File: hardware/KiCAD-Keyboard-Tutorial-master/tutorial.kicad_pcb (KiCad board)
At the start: 2 copper layers, 185.7 x 106 mm, 51 parts, among them SW0:0 CTRL, SW0:1 SUPER, SW0:2 ALT, SW0:4 SPACE, SW1:1 SHIFT, SW1:2 Z, SW1:3 X, SW1:4 C, SW2:0 CAPS, SW2:1 A, SW2:2 S, SW2:3 D, SW2:4 F, SW3:0 TAB, SW3:1 Q, SW3:2 W, SW3:3 E, SW3:4 R, SW4:0 TILDE, SW4:1 1, SW4:2 2, SW4:3 3, SW4:4 4

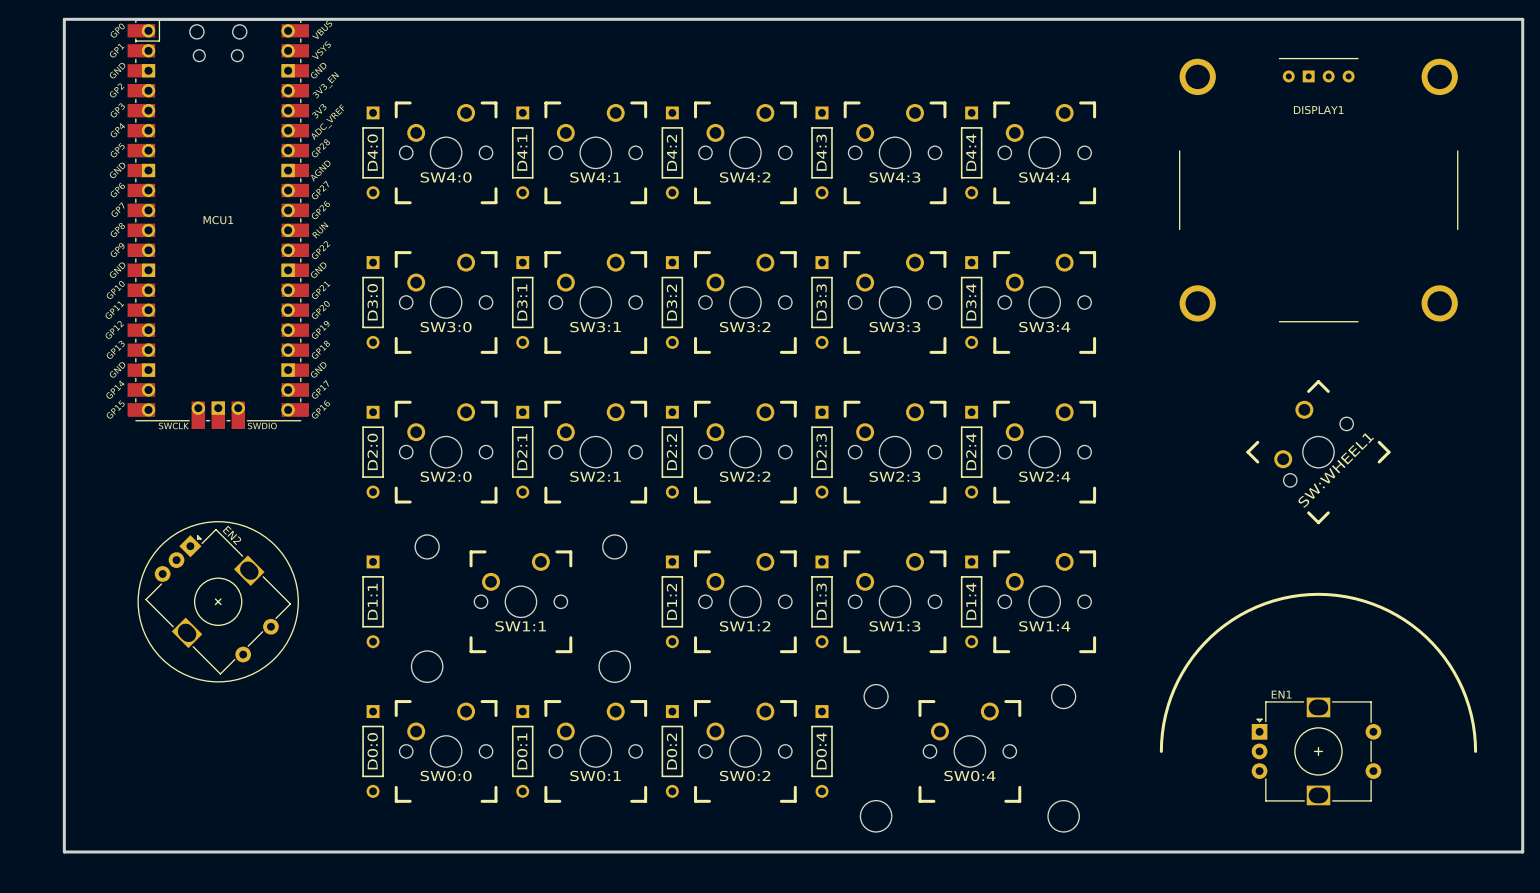
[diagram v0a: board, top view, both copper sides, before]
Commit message: pcb polished
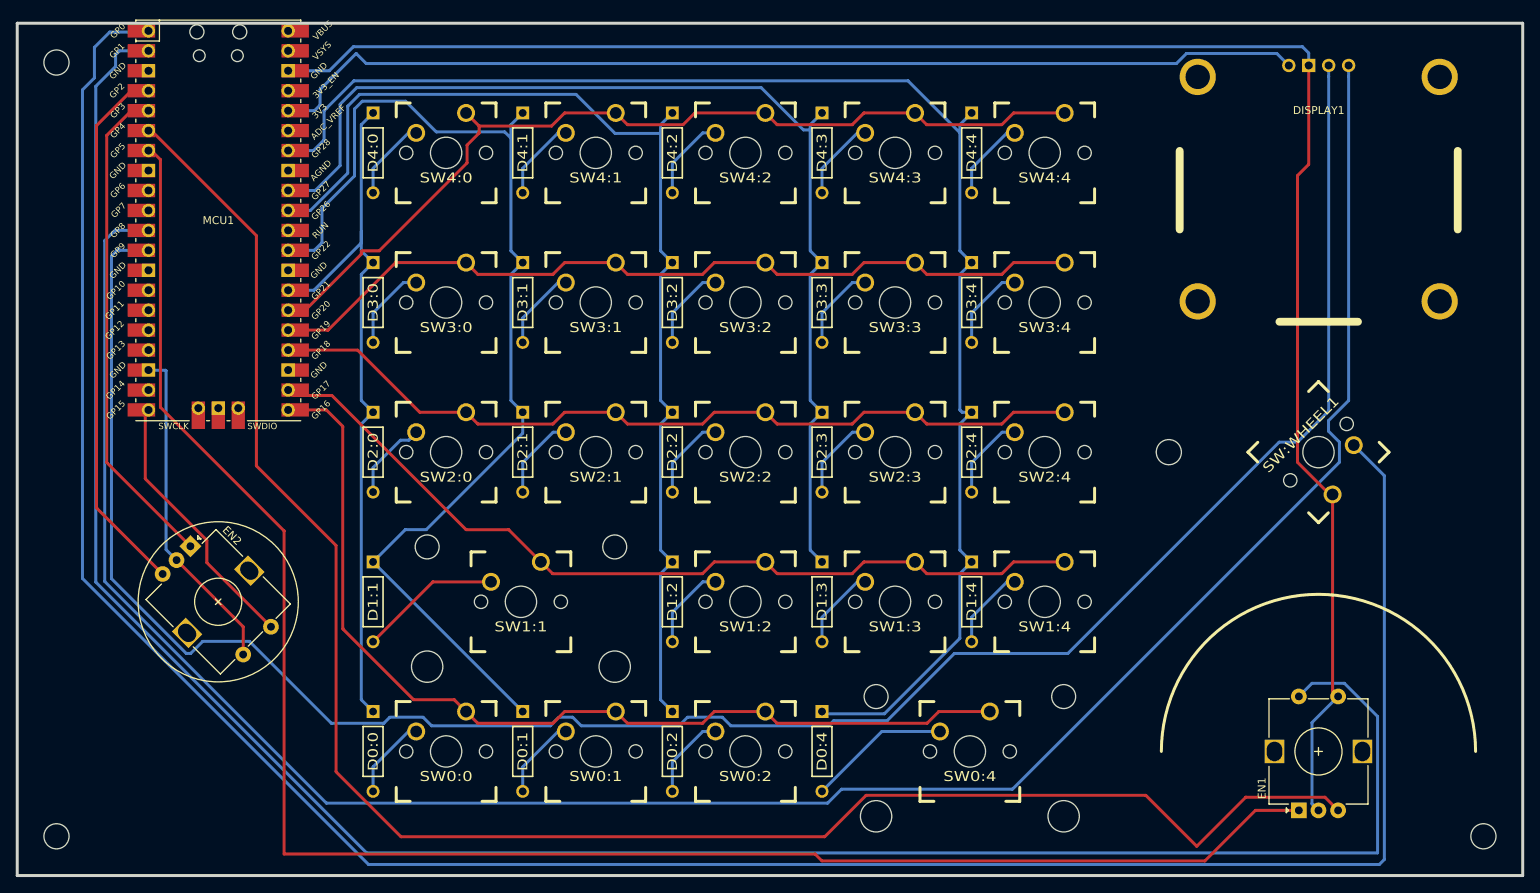
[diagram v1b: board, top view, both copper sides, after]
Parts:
- added hole1: MountingHole_3.2mm_M3, MountingHole:MountingHole_3.2mm_M3, F.Cu at (330.4, 28.5)
- added hole1: MountingHole_3.2mm_M3, MountingHole:MountingHole_3.2mm_M3, F.Cu at (512.0, 127.0)
- added hole1: MountingHole_3.2mm_M3, MountingHole:MountingHole_3.2mm_M3, F.Cu at (330.4, 127.0)
- added hole1: MountingHole_3.2mm_M3, MountingHole:MountingHole_3.2mm_M3, F.Cu at (472.0, 78.1)
- moved EN1 11.2 mm to (488.6, 123.7), turned to 90 degrees
- turned SW:WHEEL1 to 225 degrees
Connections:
- MCU1 pad 1: Net-(MCU1-Pad1) -> /SW_WHEEL
- MCU1 pad 15: /COL0 -> Net-(MCU1-Pad15)
- MCU1 pad 16: /COL1 -> Net-(MCU1-Pad16)
- MCU1 pad 17: /COL2 -> Net-(MCU1-Pad17)
- MCU1 pad 19: /COL3 -> Net-(MCU1-Pad19)
- MCU1 pad 2: Net-(MCU1-Pad2) -> /EN1_SW
- MCU1 pad 20: /COL4 -> /EN2_SW
- MCU1 pad 21: /ROW4 -> /ROW0
- MCU1 pad 22: /ROW3 -> /ROW1
- MCU1 pad 25: /ROW1 -> /ROW3
- MCU1 pad 26: /ROW0 -> /ROW4
- MCU1 pad 27: /SW_WHEEL -> /COL0
- MCU1 pad 29: Net-(MCU1-Pad29) -> /COL1
- MCU1 pad 31: /EN1_SW -> /COL2
- MCU1 pad 32: /EN2_SW -> /COL3
- MCU1 pad 34: Net-(MCU1-Pad34) -> /COL4
- MCU1 pad 4: /EN1_B -> /EN2_B
- MCU1 pad 5: /EN1_A -> /EN2_A
- MCU1 pad 6: /EN2_B -> /EN1_B
- MCU1 pad 7: /EN2_A -> /EN1_A
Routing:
- net /SW_WHEEL: track 0.00 -> 311.4 mm
- net /SDA: track 0.00 -> 288.5 mm
- net /EN1_SW: track 0.00 -> 279.9 mm
- net GND: track 0.00 -> 275.1 mm
- net /SCL: track 0.00 -> 273.2 mm
- net /EN1_B: track 0.00 -> 230.9 mm
- net /EN1_A: track 0.00 -> 229.1 mm
- net /COL4: track 0.00 -> 187.7 mm
- net /COL2: track 0.00 -> 141.7 mm
- net /COL1: track 0.00 -> 141.7 mm
- net /COL3: track 0.00 -> 139.6 mm
- net VCC: track 0.00 -> 133.2 mm
- net /ROW0: track 0.00 -> 124.0 mm
- net /ROW4: track 0.00 -> 117.3 mm
- net /ROW1: track 0.00 -> 111.6 mm
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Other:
- board size 185.7 x 106 mm -> 191.6 x 108.5 mm
